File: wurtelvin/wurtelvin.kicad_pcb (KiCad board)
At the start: 2 copper layers, 40 x 130 mm, 92 parts, among them J1 BATT, J10 FIN_TOP, J2 FRONT, J3 MIRRORS, J4 REAR TURNERS, J5 REAR, J6 BTN_BRK, J7 BTN_HANDLE, J8 FIN_REAR, J9 FIN_FRONT, SW1 SW_DPDT_x2, SW2 DAYLIGHT, SW4 REAR, U1 STM32F103C8Tx, U10 XL1509-5.0, U2 AL8860WT, U3 AL8860WT, U4 AL8860WT, U5 AL8860WT, U6 AL8860WT, U7 AL8860WT, U8 AL8860WT, U9 XL1509-3.3, Y1 8MHz

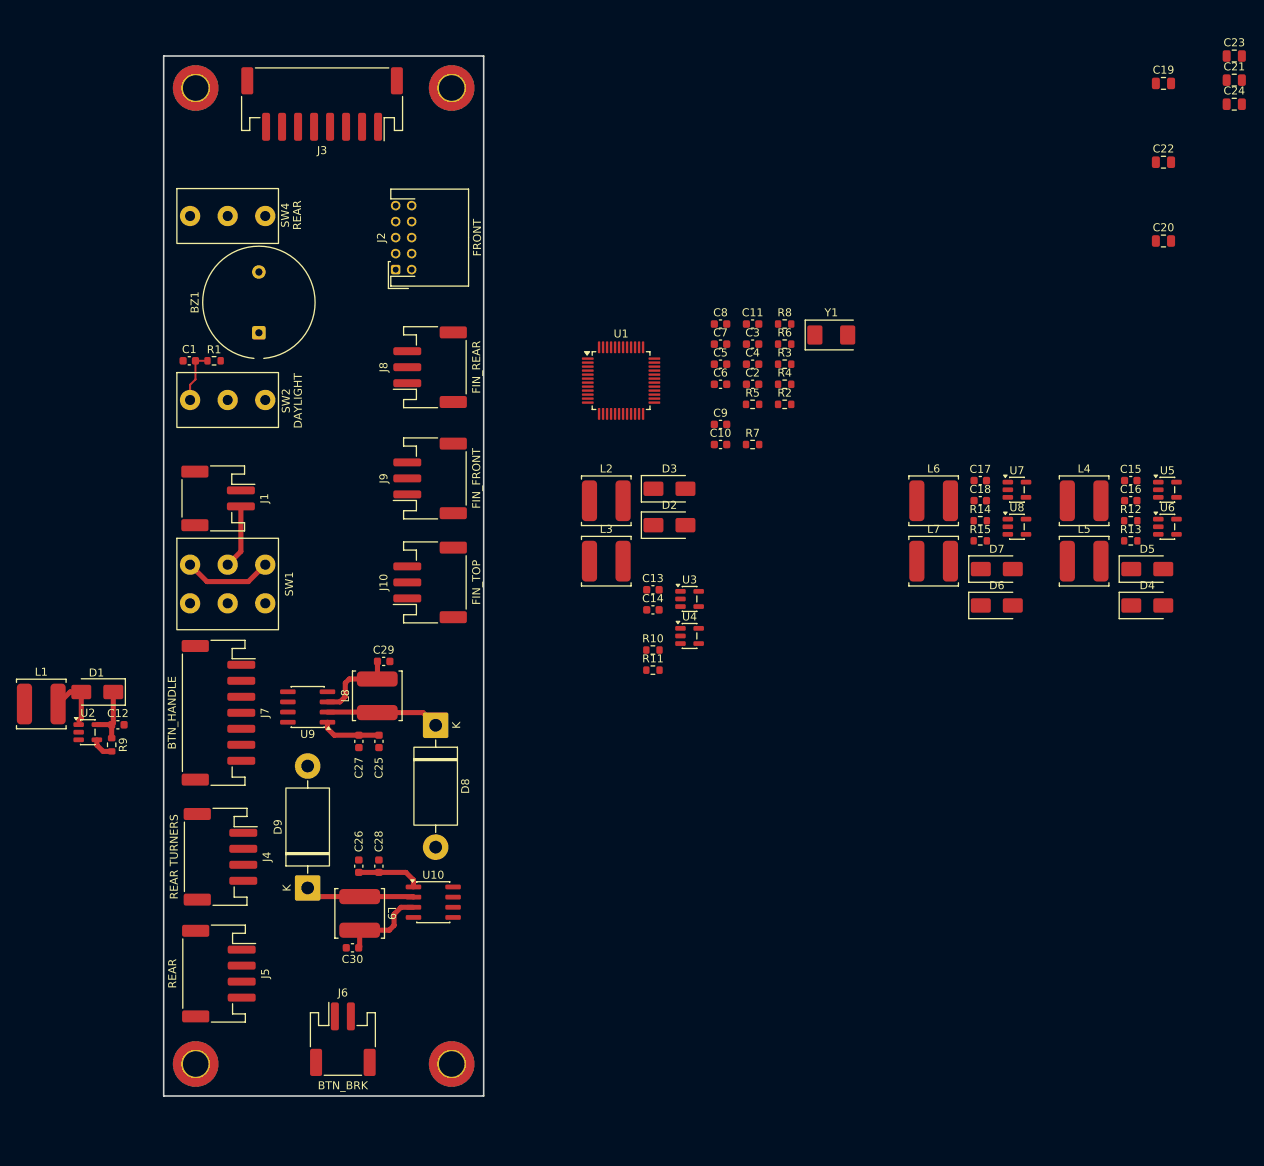
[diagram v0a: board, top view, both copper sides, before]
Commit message: furhter pcb layout
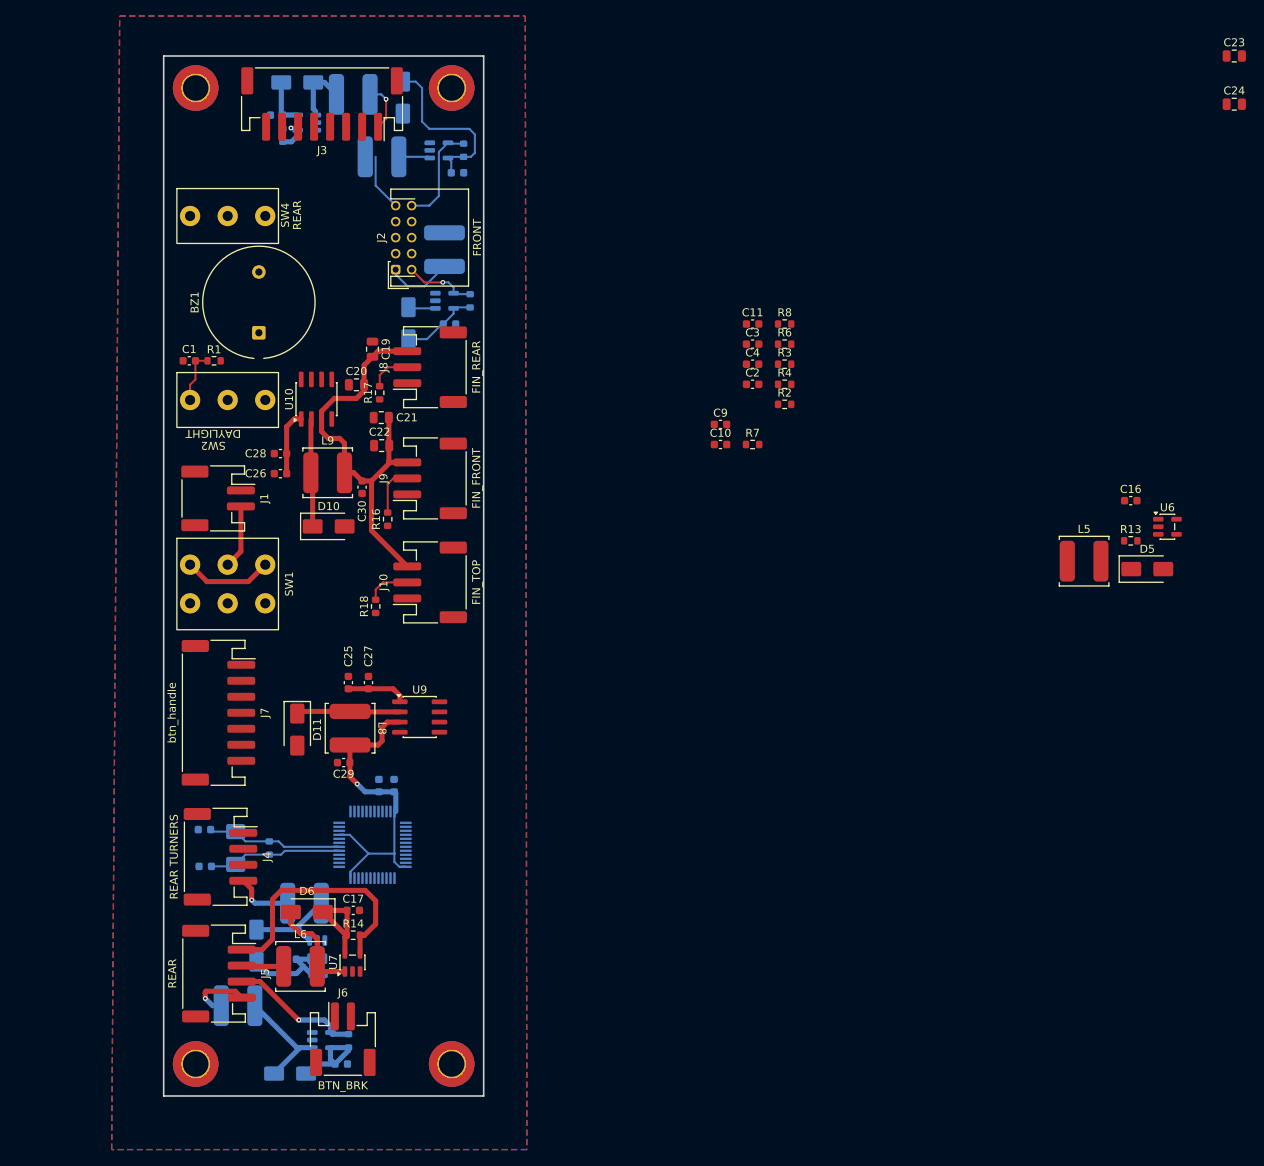
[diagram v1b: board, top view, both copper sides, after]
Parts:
- removed D8, D9: 1N5820, Diode_THT:D_DO-201AD_P15.24mm_Horizontal
- added D10: SS32, Diode_SMD:D_SMA, F.Cu at (135.6, 83.8)
- added D11: SS32, Diode_SMD:D_SMA, F.Cu at (131.7, 109.2)
- added R16: 300, Resistor_SMD:R_0603_1608Metric, F.Cu at (143.0, 82.9)
- added R17: 300, Resistor_SMD:R_0603_1608Metric, F.Cu at (142.0, 67.1)
- added R18: 300, Resistor_SMD:R_0603_1608Metric, F.Cu at (141.5, 93.8)
- C12, C13, C14, C15, C18, C5, C6, C7, C8, D1, D2, D3, D4, D7, L1, L2, L3, L4, L7, R10, R11, R12, R15, R5, R9, U1, U2, U3, U4, U5, U8, Y1: moved to B.Cu
- J7: value BTN_HANDLE -> btn_handle
- moved C15 120.9 mm to (130.8, 137.9), turned to 180 degrees
- moved U5 120.8 mm to (134.2, 136.7), turned to -90 degrees
- moved D4 119.2 mm to (126.6, 136.2), turned to 90 degrees
- moved R12 116.3 mm to (134.3, 139.8)
- moved C21 114.7 mm to (142.2, 70.2)
- moved L4 109.7 mm to (132.6, 130.9)
- moved D7 108.5 mm to (130.8, 152.2), turned to 180 degrees
- moved U8 108.1 mm to (134.7, 148.0)
- moved C18 106.5 mm to (137.2, 151.0)
- moved C19 104.3 mm to (141.1, 61.6), turned to -90 degrees
- moved C22 103.9 mm to (142.2, 73.7)
- moved L7 103.2 mm to (124.3, 143.7)
- moved C20 102.5 mm to (139.1, 66.1)
- moved U7 101.9 mm to (138.6, 138.3), turned to 90 degrees
- moved R15 100.7 mm to (138.1, 148.1), turned to 90 degrees
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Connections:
- net /front_lights/CTRL_DL renamed /CTRL_DL
- net /front_lights/CTRL_FH renamed /CTRL_FH
- net /front_lights/CTRL_FL renamed /CTRL_FL
- net /rear_lights/CTRL_BRK renamed /CTRL_BRK
- net /rear_lights/CTRL_REAR renamed /CTRL_REAR
- net /turning_lights/CTRL_TLL renamed /CTRL_TLL
- net /turning_lights/CTRL_TLR renamed /CTRL_TLR
- J10 pad 2: /fin_lights/FT_DATA -> Net-(J10-Pin_2)
- J8 pad 2: /fin_lights/FR_DATA -> Net-(J8-Pin_2)
- J9 pad 2: /fin_lights/FF_DATA -> Net-(J9-Pin_2)
- L1 pad 1: /front_lights/DL- -> /DL-
- L2 pad 1: /front_lights/FH- -> /FH-
- L3 pad 1: /front_lights/FL- -> /FL-
- L4 pad 1: /turning_lights/TLR- -> /TLR-
- L5 pad 1: /turning_lights/TLL- -> /TLL-
- L6 pad 1: /rear_lights/REAR- -> /REAR-
- L7 pad 1: /rear_lights/BRK- -> /BRK-
- R10 pad 2: /front_lights/FH+ -> /FH+
- R11 pad 2: /front_lights/FL+ -> /FL+
- R12 pad 2: /turning_lights/TLR+ -> /TLR+
- R13 pad 2: /turning_lights/TLL+ -> /TLL+
- R14 pad 2: /rear_lights/REAR+ -> /REAR+
- R15 pad 2: /rear_lights/BRK+ -> /BRK+
- R9 pad 2: /front_lights/DL+ -> /DL+
- U2 pad 4: /front_lights/DL+ -> /DL+
- U3 pad 4: /front_lights/FH+ -> /FH+
- U4 pad 4: /front_lights/FL+ -> /FL+
- U5 pad 4: /turning_lights/TLR+ -> /TLR+
- U6 pad 4: /turning_lights/TLL+ -> /TLL+
- U7 pad 4: /rear_lights/REAR+ -> /REAR+
- U8 pad 4: /rear_lights/BRK+ -> /BRK+
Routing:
- net +BATT: track 35.1 -> 104.5 mm
- net +5V: track 11.0 -> 52.8 mm
- net /REAR+: track 0.00 -> 31.0 mm
- net +3V3: track 10.6 -> 41.1 mm, vias 0 -> 1
- net /OSC_OUT: track 0.00 -> 17.0 mm
- net /OSC_IN: track 0.00 -> 16.8 mm
- net /BRK+: track 0.00 -> 16.5 mm, vias 0 -> 1
- net Net-(D7-A): track 0.00 -> 13.9 mm
- net /FH+: track 0.00 -> 13.0 mm
- net Net-(D6-A): track 0.00 -> 12.7 mm
- net Net-(D4-A): track 0.00 -> 11.7 mm
- net /FL+: track 0.00 -> 8.99 mm, vias 0 -> 1
- net /FL-: track 0.00 -> 8.36 mm
- net /BRK-: track 0.00 -> 8.10 mm, vias 0 -> 1
- net /TLR-: track 0.00 -> 7.50 mm, vias 0 -> 1
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- added copper zone on B.Cu, net GND
- added copper zone on F.Cu, net GND
